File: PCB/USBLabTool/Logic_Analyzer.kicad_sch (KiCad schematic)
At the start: 20 parts, among them U18 74HC245N, U19 74HC245N

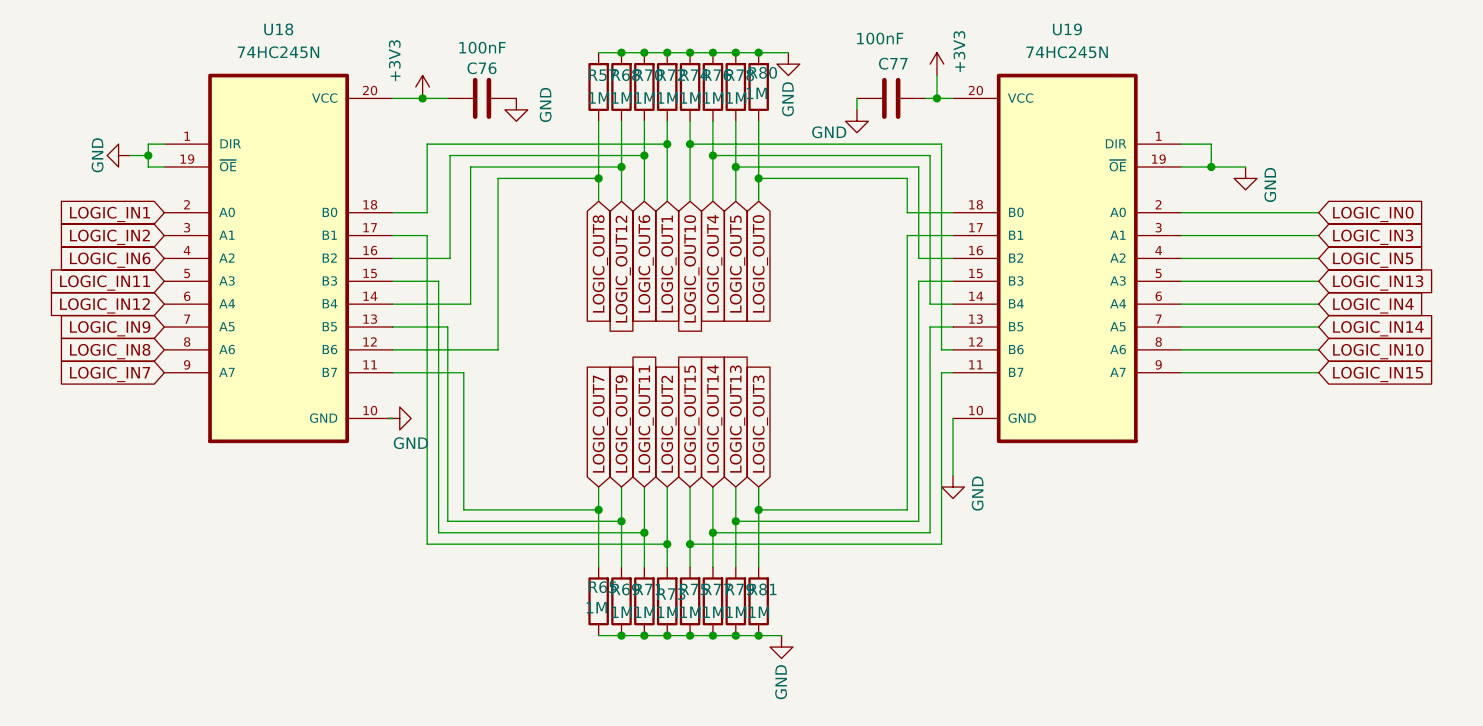
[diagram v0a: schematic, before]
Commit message: minor fixes
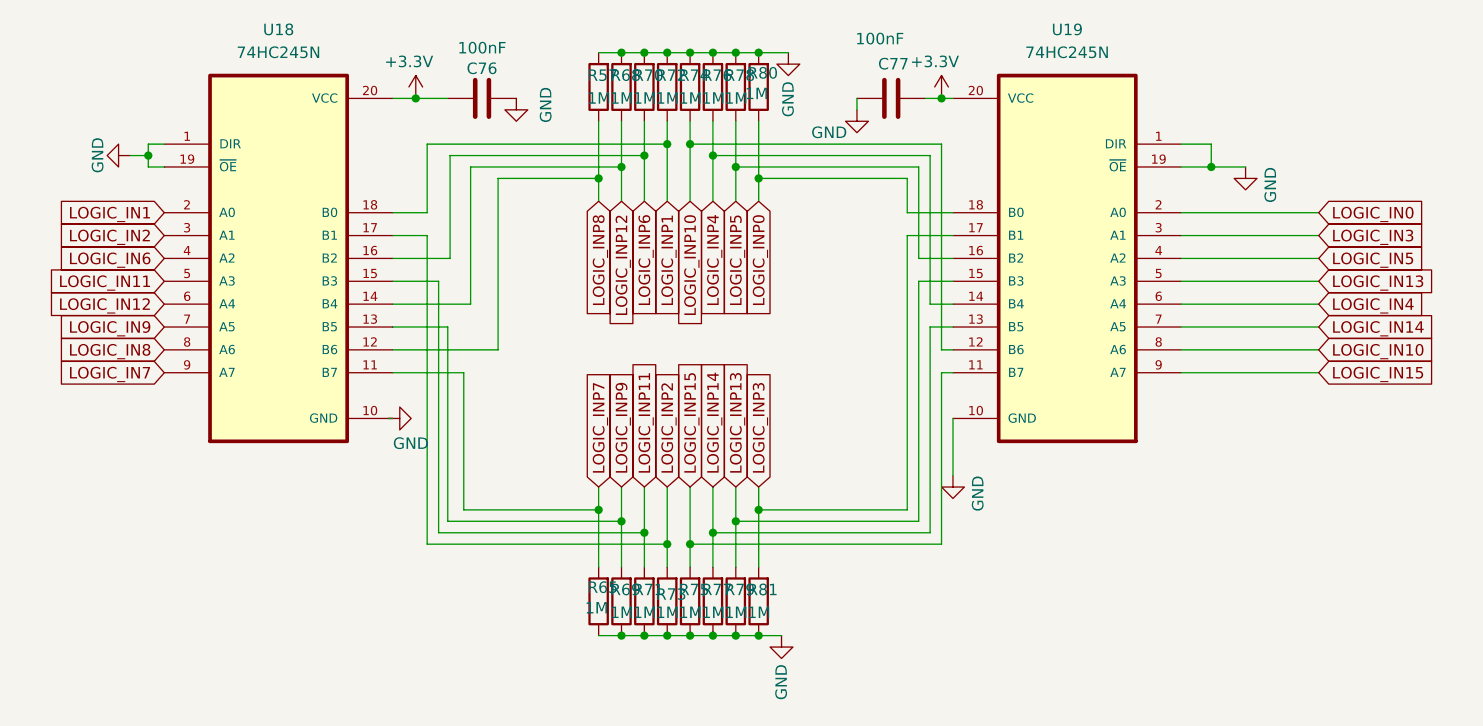
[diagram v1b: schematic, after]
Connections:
- net +3V3 renamed +3.3V
- net LOGIC_OUT0 renamed LOGIC_INP0
- net LOGIC_OUT1 renamed LOGIC_INP1
- net LOGIC_OUT10 renamed LOGIC_INP10
- net LOGIC_OUT11 renamed LOGIC_INP11
- net LOGIC_OUT12 renamed LOGIC_INP12
- net LOGIC_OUT13 renamed LOGIC_INP13
- net LOGIC_OUT14 renamed LOGIC_INP14
- net LOGIC_OUT15 renamed LOGIC_INP15
- net LOGIC_OUT2 renamed LOGIC_INP2
- net LOGIC_OUT3 renamed LOGIC_INP3
- net LOGIC_OUT4 renamed LOGIC_INP4
- net LOGIC_OUT5 renamed LOGIC_INP5
- net LOGIC_OUT6 renamed LOGIC_INP6
- net LOGIC_OUT7 renamed LOGIC_INP7
- net LOGIC_OUT8 renamed LOGIC_INP8
- net LOGIC_OUT9 renamed LOGIC_INP9
